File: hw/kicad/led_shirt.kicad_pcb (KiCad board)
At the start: 2 copper layers, 20.6 x 20.6 mm, 18 parts, among them J1 10103593-0001LF, Q1 MOSFET_N, SW1 SW_PUSH, U1 PIC12F1822, U2 MCP73831

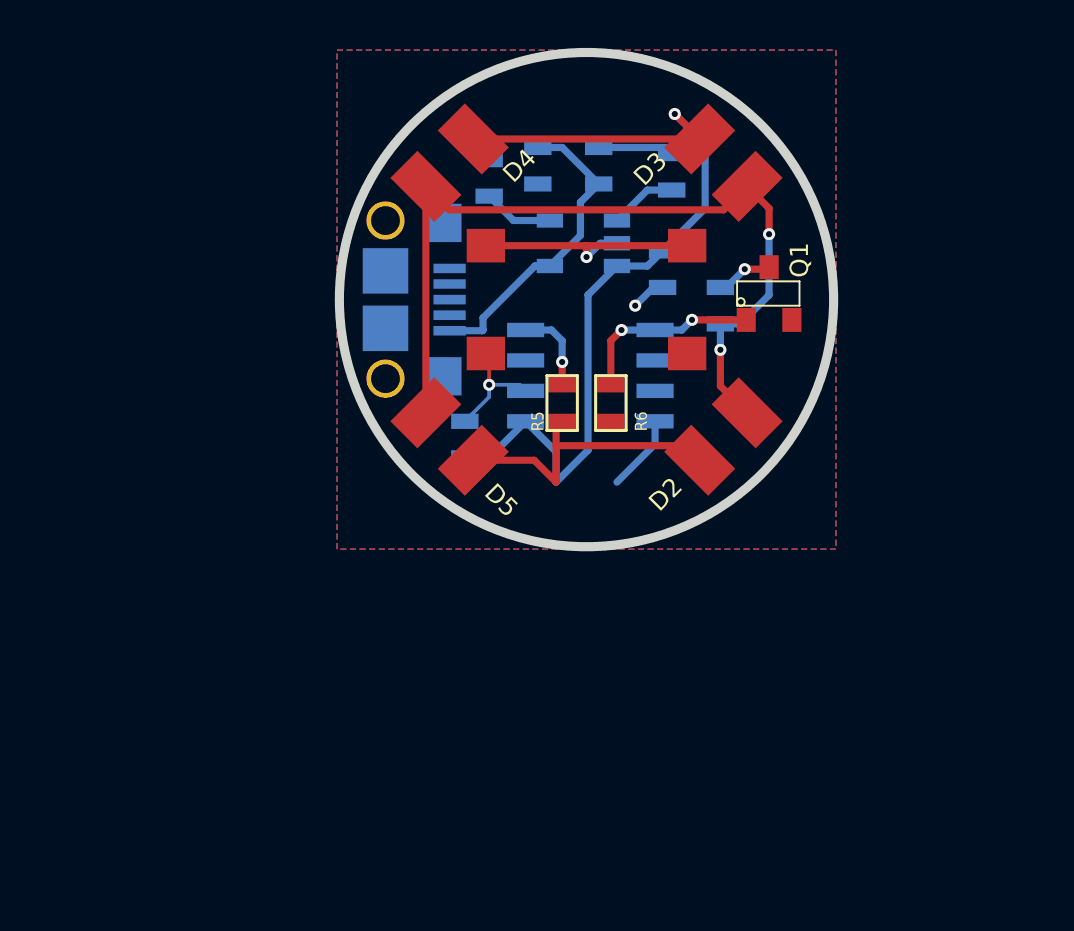
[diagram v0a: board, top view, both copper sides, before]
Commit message: update sch
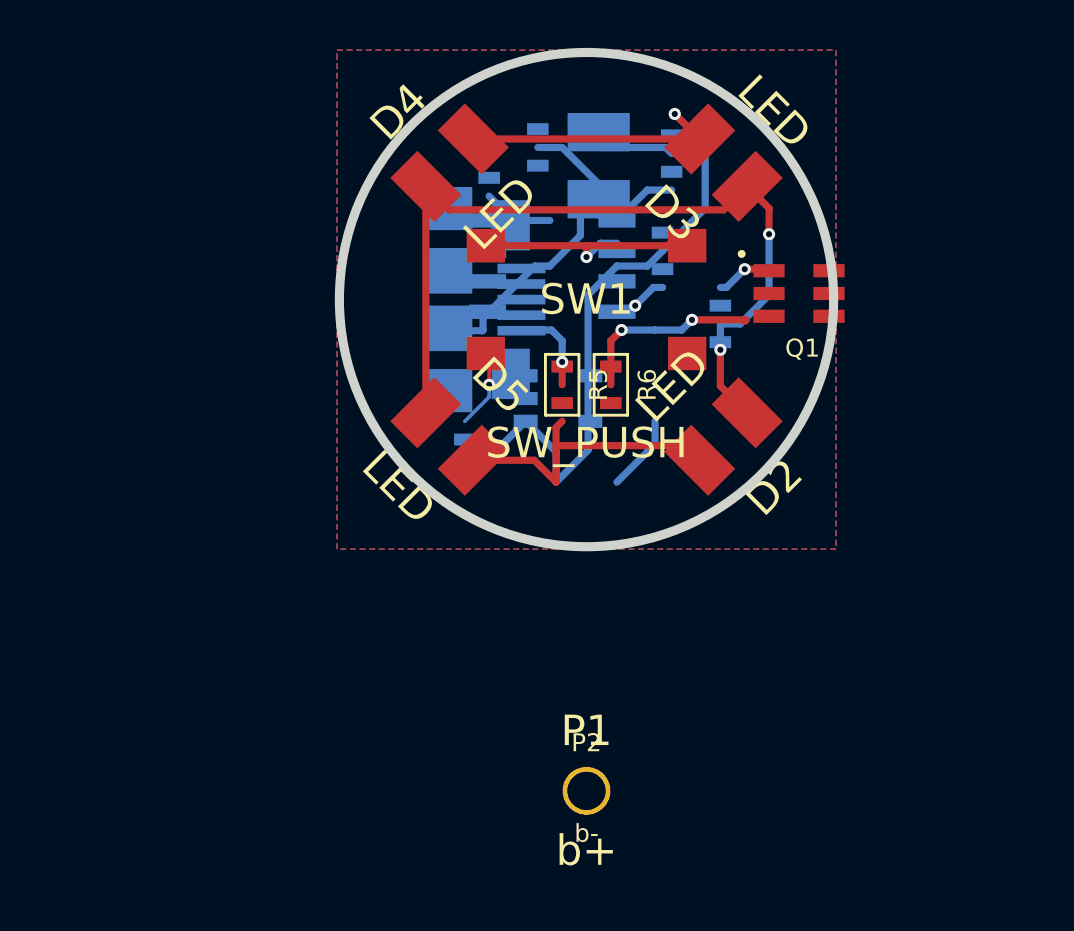
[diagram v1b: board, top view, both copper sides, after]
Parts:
- added P1: b+, noah:noah_hole_1, F.Cu at (153.7, 117.0)
- added P2: b-, kicadlib:med_test_hole, F.Cu at (153.7, 117.0)
- C1, C2, R1, R2, R3, R4, R5, R6: footprint SM0603 -> kicadlib:SMD_0603_R
- D1: footprint SM0603 -> kicadlib:plcc2
- D2, D3, D4, D5: footprint plcc2 -> kicadlib:plcc2
- J1: footprint 10118193-0001LF -> kicadlib:usb_micro_b_smt
- Q1: value MOSFET_N -> PN_MOSFET_DUAL; footprint SOT23 -> kicadlib:SMD_SOT23-6
- SW1: footprint SW_PB_4PIN_SMT_real -> noah:SW_PB_4PIN_SMT_real
- U1: footprint MCP73831 -> noah:PIC12F1822-SOIC-8
- U2: footprint PIC12F1822-SOIC-8 -> kicadlib:MCP73831
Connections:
- net Net-(Q1-Pad2) renamed Q2_S
- Q1 pad 1: Net-(Q1-Pad1) -> Q1_G
- Q1 pad 3: vbat -> Q2_G
- R1 pad 1: Net-(Q1-Pad1) -> vbat
- R1 pad 2: GND -> Q2_G
- R2 pad 2: Net-(Q2-Pad3) -> Q1_D
- R4 pad 1: Net-(Q2-Pad1) -> Q1_G
- SW1 pad 1: vbat -> GND
- SW1 pad 2: Net-(Q1-Pad1) -> Q2_G
- U1 pad 2: Net-(Q1-Pad1) -> Q2_G
- U1 pad 5: Net-(Q2-Pad1) -> Q1_G
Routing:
- net GND: track 6.56 -> 18.7 mm, vias 2 -> 1
- net vbat: track 42.5 -> 31.2 mm, vias 2 -> 1
- net (no net): track 3.20 -> 13.3 mm, vias 0 -> 3
- net Net-(Q2-Pad1): track 7.67 -> 0.00 mm, vias 2 -> 0
- net Net-(D1-Pad2): track 33.4 -> 40.9 mm, vias 0 -> 2
- net mclr: track 7.89 -> 1.46 mm, vias 0 -> 1
- net Net-(Q1-Pad1): track 6.28 -> 0.00 mm, vias 1 -> 0
- net Q1_G: track 0.00 -> 5.99 mm, vias 0 -> 1
- net Net-(R6-Pad2): track 13.6 -> 18.5 mm
- net Net-(R5-Pad1): track 4.07 -> 0.95 mm, vias 3 -> 1
- net Net-(U1-Pad3): track 2.98 -> 0.00 mm
- net vbus: track 8.07 -> 5.14 mm
- net Net-(D5-Pad2): track 2.47 -> 0.00 mm
- net Q2_G: track 0.00 -> 1.36 mm
- net Q2_S: track 1.80 -> 2.81 mm

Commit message: more components
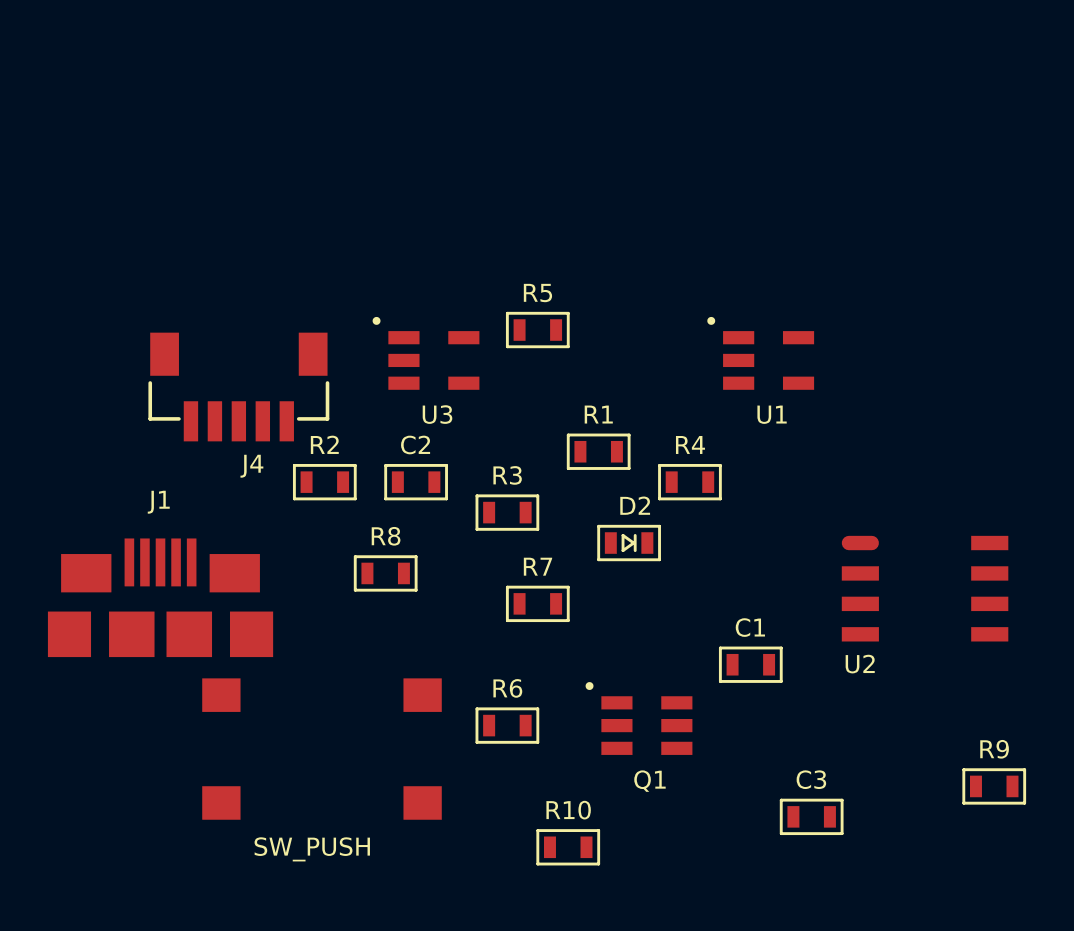
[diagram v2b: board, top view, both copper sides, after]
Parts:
- removed D1, D3, D4, D5: LED, kicadlib:plcc2
- removed P1: b+, noah:noah_hole_1
- removed P2: b-, kicadlib:med_test_hole
- added C3: 4.7µF, kicadlib:SMD_0603_R, F.Cu at (163.8, 118.1)
- added J4: 5_PIN_HDR, kicadlib:SMD_JST_5_PIN_VERT, F.Cu at (137.2, 101.6)
- added R10: 3.3kΩ, kicadlib:SMD_0603_R, F.Cu at (153.7, 119.4)
- added R7: 10K, kicadlib:SMD_0603_R, F.Cu at (152.4, 109.2)
- added R8: 10K, kicadlib:SMD_0603_R, F.Cu at (146.1, 108.0)
- added R9: 3.3kΩ, kicadlib:SMD_0603_R, F.Cu at (171.4, 116.8)
- added U3: MCP73831, kicadlib:SMD_SOT23-5, F.Cu at (146.1, 99.1)
- C1: value 4.7µF -> 1.0µF; moved to F.Cu
- C2, J1, R1: moved to F.Cu
- D2: footprint kicadlib:plcc2 -> kicadlib:SMD_0603_LED
- R2: value 0Ω -> 10kΩ; moved to F.Cu
- R3, R4: value 10K -> 10kΩ; moved to F.Cu
- R5: value 3.3kΩ -> 0Ω
- R6: value 3.3kΩ -> 10kΩ
- SW1: footprint noah:SW_PB_4PIN_SMT_real -> kicadlib:spst_pushbutton_smd
- U1: value PIC12F1822 -> AP3012; footprint noah:PIC12F1822-SOIC-8 -> kicadlib:SMD_SOT23-5; moved to F.Cu
- U2: value MCP73831 -> PIC12F1822; footprint kicadlib:MCP73831 -> kicadlib:SMD_SOIC-8; moved to F.Cu
- moved C1 23.0 mm to (161.3, 111.8), turned to 0 degrees
- moved SW1 22.5 mm to (138.4, 113.0)
- moved Q1 19.1 mm to (154.9, 114.3)
- moved J1 18.5 mm to (135.9, 110.5), turned to 0 degrees
- moved U2 14.9 mm to (165.1, 106.7), turned to 0 degrees
- moved R2 14.1 mm to (143.5, 104.1), turned to 0 degrees
- moved R6 13.9 mm to (151.1, 114.3), turned to 0 degrees
- moved C2 13.0 mm to (147.3, 104.1), turned to 0 degrees
- moved R1 11.9 mm to (154.9, 102.9), turned to 0 degrees
- moved U1 7.74 mm to (160.0, 99.1), turned to 0 degrees
- moved R4 7.38 mm to (158.8, 104.1), turned to 0 degrees
- moved D2 5.46 mm to (156.2, 106.7), turned to 0 degrees
- moved R3 3.97 mm to (151.1, 105.4), turned to 0 degrees
- moved R5 3.06 mm to (152.4, 97.8), turned to 0 degrees
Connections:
- C1 pad 1: vbus -> /+12v
- C2 pad 1: vbat -> /vbus
- D2 pad 1: vbat -> /vbus
- D2 pad 2: Net-(D1-Pad2) -> Net-(D2-Pad2)
- J1 pad 1: vbus -> /vbus
- J1 pad 2: icspdat -> Net-(J1-Pad2)
- J1 pad 3: mclr -> Net-(J1-Pad3)
- J1 pad 4: icspclk -> Net-(J1-Pad4)
- Q1 pad 1: Q1_G -> /led_cntrl
- Q1 pad 2: Q2_S -> /lps
- Q1 pad 3: Q2_G -> /~lps_enable
- Q1 pad 4: vbat -> /vbat
- Q1 pad 6: Q1_D -> Net-(Q1-Pad6)
- R1 pad 1: vbat -> /+12v
- R1 pad 2: Q2_G -> Net-(R1-Pad2)
- R2 pad 1: Net-(D1-Pad2) -> Net-(R1-Pad2)
- R2 pad 2: Q1_D -> GND
- R3 pad 1: mclr -> /vbat
- R3 pad 2: vbat -> /~lps_enable
- R4 pad 1: Q1_G -> /lps
- R4 pad 2: GND -> /batt_sns
- R5 pad 1: Net-(R5-Pad1) -> /led-
- R5 pad 2: GND -> Net-(Q1-Pad6)
- R6 pad 1: Net-(D5-Pad2) -> /batt_sns
- R6 pad 2: Net-(R6-Pad2) -> GND
- SW1 pad 2: Q2_G -> /~lps_enable
- U1 pad 1: Q2_S -> Net-(D1-Pad2)
- U1 pad 2: Q2_G -> GND
- U1 pad 3: Net-(U1-Pad3) -> Net-(R1-Pad2)
- U1 pad 4: mclr -> /lps
- U1 pad 5: Q1_G -> /vbat
- U2 pad 1: Net-(R6-Pad2) -> /lps
- U2 pad 2: GND -> /~lps_enable
- U2 pad 3: vbat -> /batt_sns
- U2 pad 4: vbus -> /mclr
- U2 pad 5: Net-(R5-Pad1) -> /led_cntrl
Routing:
- net Net-(D1-Pad2): track 40.9 -> 0.00 mm, vias 2 -> 0
- net vbat: track 31.2 -> 0.00 mm, vias 1 -> 0
- net GND: track 18.7 -> 0.00 mm, vias 1 -> 0
- net Net-(R6-Pad2): track 18.5 -> 0.00 mm
- net (no net): track 13.3 -> 0.00 mm, vias 3 -> 0
- net Q1_G: track 5.99 -> 0.00 mm, vias 1 -> 0
- net vbus: track 5.14 -> 0.00 mm
- net Q2_S: track 2.81 -> 0.00 mm
- net mclr: track 1.46 -> 0.00 mm, vias 1 -> 0
- net Q2_G: track 1.36 -> 0.00 mm
- net Net-(R5-Pad1): track 0.95 -> 0.00 mm, vias 1 -> 0
- removed copper zone on B.Cu, net GND
- removed copper zone on F.Cu, net GND
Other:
- board outline removed
- board text removed: "+"
- board text removed: "-"
- board text removed: "c"
- board text removed: "d"
- board text removed: "git.io/FEFjUw v2.0"
- board text removed: "ledshirt"
- board text removed: "m"
